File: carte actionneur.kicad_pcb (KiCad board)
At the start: 2 copper layers, 106 x 136.7 mm, 88 parts, among them J1 Conn_01x03_Pin, J10 Conn_01x03_Pin, J11 Conn_01x02, J12 Conn_01x02_Pin, J13 Conn_01x02_Pin, J14 Conn_01x02_Pin, J15 Conn_01x02, J16 Conn_01x02_Pin, J17 Conn_01x04_Pin, J18 Conn_01x02_Pin, J19 Conn_01x04_Pin, J2 Conn_01x02, J20 Conn_01x02_Pin, J21 Conn_01x08_Pin, J22 Conn_01x02_Pin, J23 Conn_01x02_Pin, J24 Conn_01x02_Pin, J25 Conn_01x03_Pin, J26 Conn_01x03_Pin, J27 Conn_01x03_Pin, J28 Conn_01x02_Pin, J3 Conn_01x04_Pin, J4 Conn_01x02_Pin, J5 Connecteur Programmation, J6 Conn_01x08_Pin, J7 Conn_01x03_Pin, J8 Conn_01x03_Pin, J9 Conn_01x03_Pin, Q1 Q_NMOS_GDS, Q2 QM6006D, Q3 QM6006D, Q4 QM6006D, U1 MEGA_PRO_EMBED_CH340G___ATMEG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, U2 YAAJ_DCDC_StepDown_LM2596, U3 ZXBM5210-SP, U4 YAAJ_DCDC_StepDown_LM2596, U5 YAAJ_DCDC_StepDown_LM2596, U7 ZXBM5210-SP

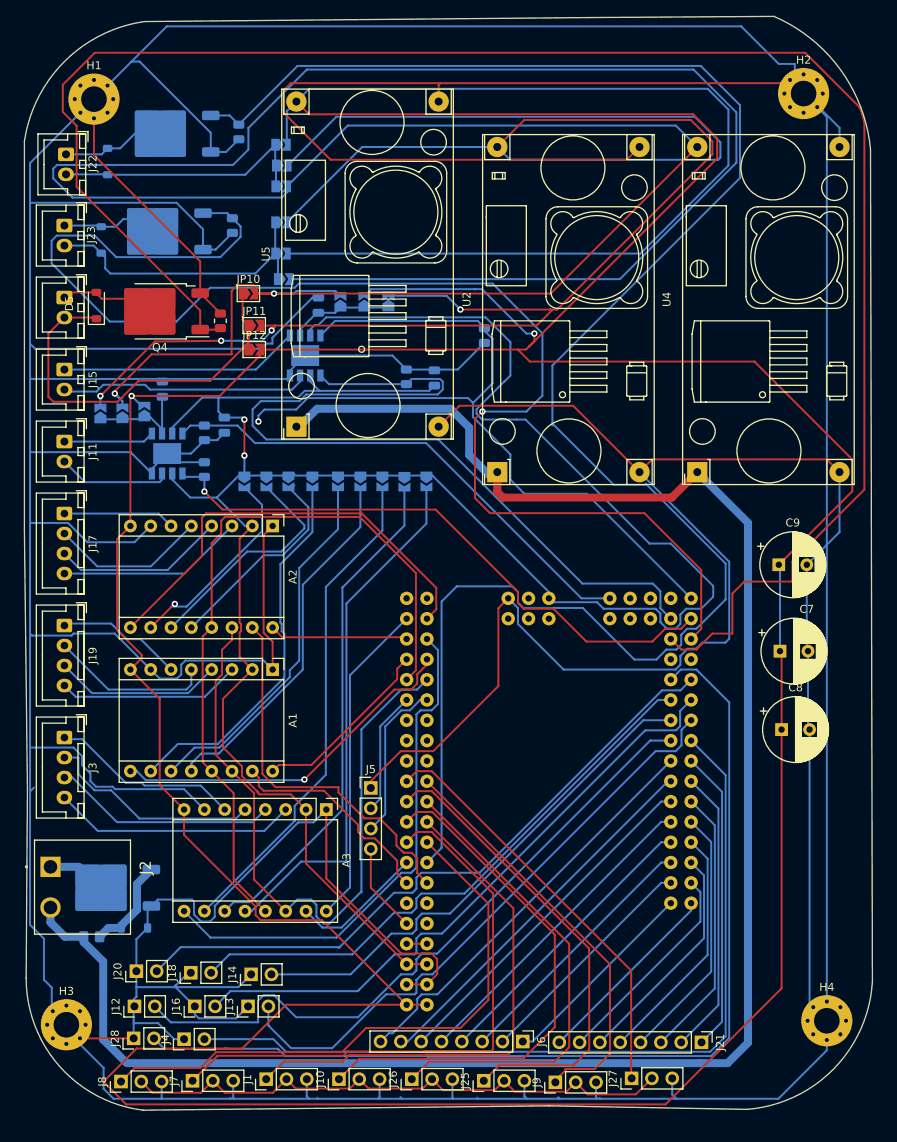
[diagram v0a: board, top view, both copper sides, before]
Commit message: PCB fini
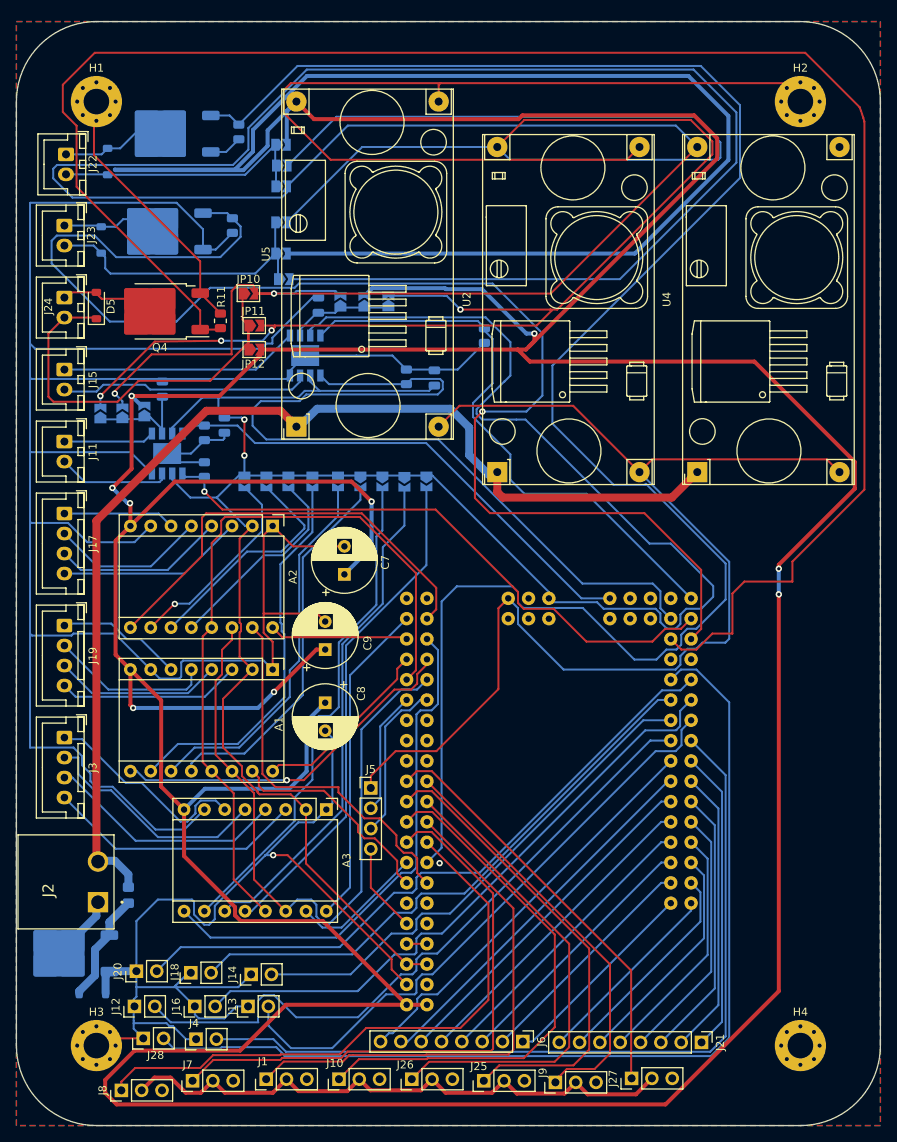
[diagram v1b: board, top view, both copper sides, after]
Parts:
- moved C9 57.7 mm to (139.6, 117.5), turned to 90 degrees
- moved C8 57.1 mm to (139.6, 124.1), turned to -90 degrees
- moved C7 55.3 mm to (142.0, 108.1), turned to 90 degrees
- moved D1 9.74 mm to (110.5, 160.5)
- moved Q1 9.74 mm to (107.6, 155.5)
- moved J2 7.40 mm to (111.2, 149.1), turned to 90 degrees
- moved R1 6.94 mm to (115.0, 148.2), turned to -90 degrees
- moved H3 4.56 mm to (111.0, 167.0)
- moved H4 4.53 mm to (199.0, 167.0)
- moved J4 1.50 mm to (123.5, 166.2)
- moved J28 1.20 mm to (116.9, 166.1)
- moved J8 1.10 mm to (114.1, 172.6)
- moved H2 1.08 mm to (199.0, 49.0)
- moved H1 0.43 mm to (111.0, 49.0)
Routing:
- net GND: track 1254.7 -> 791.3 mm, vias 0 -> 2
- net 12V Mot: track 650.8 -> 812.7 mm, vias 2 -> 9
- net +24V: track 238.8 -> 141.5 mm
- net FWD1: track 101.0 -> 72.3 mm, vias 1 -> 0
- net Net-(J2-Pin_1): track 14.8 -> 18.2 mm
- net Net-(A3-MS3): track 66.2 -> 62.9 mm
- net Net-(A3-2B): track 23.8 -> 26.5 mm
- net Net-(A3-1A): track 28.1 -> 30.0 mm
- net Net-(A3-2A): track 27.4 -> 29.3 mm
- net Net-(A1-MS3): track 45.5 -> 47.4 mm
- net Net-(A3-1B): track 30.5 -> 32.3 mm
- net Net-(D1-K): track 12.0 -> 13.8 mm
- net 5VServo: track 71.9 -> 73.6 mm
- net Capt8: track 125.9 -> 124.2 mm
- net Capt1: track 105.4 -> 103.9 mm
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- added copper zone on B.Cu, net GND
- added copper zone on F.Cu, net GND
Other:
- board size 106 x 136.7 mm -> 108 x 138 mm
